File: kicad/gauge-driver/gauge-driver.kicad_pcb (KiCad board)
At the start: 2 copper layers, 18 parts, among them J1 Conn_01x02_Socket, U1 ESP32-WROOM-32E, U2 SN65HVD230, U3 LM2675M-3.3, Y1 Crystal

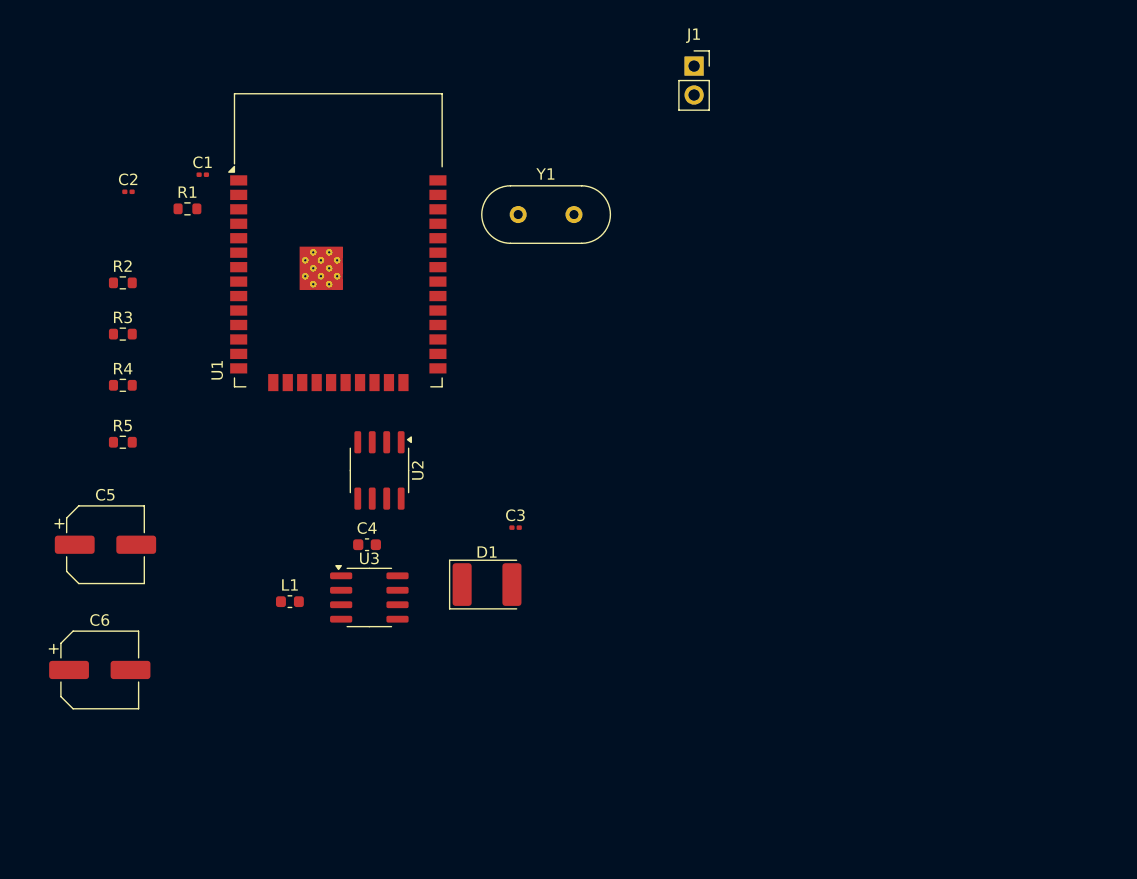
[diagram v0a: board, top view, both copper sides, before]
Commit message: kicad
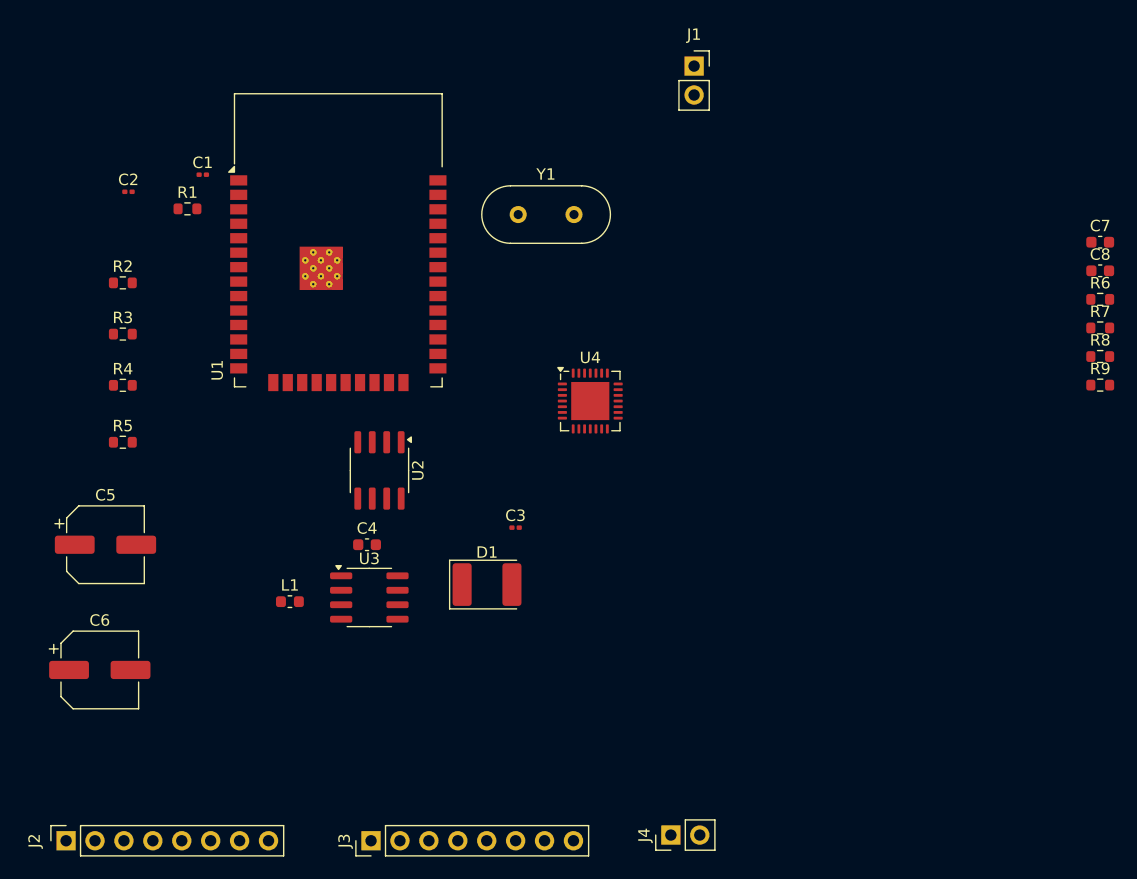
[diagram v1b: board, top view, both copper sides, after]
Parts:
- added C7: 4.7uF, Capacitor_SMD:C_0603_1608Metric, F.Cu at (106.2, 41.4)
- added C8: 4.7uF, Capacitor_SMD:C_0603_1608Metric, F.Cu at (106.2, 43.9)
- added J2: Conn_01x08, Connector_PinSocket_2.54mm:PinSocket_1x08_P2.54mm_Vertical, F.Cu at (15.3, 94.0)
- added J3: Conn_01x08, Connector_PinHeader_2.54mm:PinHeader_1x08_P2.54mm_Vertical, F.Cu at (42.1, 94.0)
- added J4: Conn_01x02_Socket, Connector_PinHeader_2.54mm:PinHeader_1x02_P2.54mm_Vertical, F.Cu at (68.5, 93.5)
- added R6: 10K, Resistor_SMD:R_0603_1608Metric, F.Cu at (106.2, 46.5)
- added R7: 2K, Resistor_SMD:R_0603_1608Metric, F.Cu at (106.2, 49.0)
- added R8: 22.1K, Resistor_SMD:R_0603_1608Metric, F.Cu at (106.2, 51.5)
- added R9: 47.5K, Resistor_SMD:R_0603_1608Metric, F.Cu at (106.2, 54.0)
- added U4: CP2102N-Axx-xQFN28, Package_DFN_QFN:QFN-28-1EP_5x5mm_P0.5mm_EP3.35x3.35mm, F.Cu at (61.4, 55.4)
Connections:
- C6 pad 1: /Vout_3v3 -> VDD33
- L1 pad 2: /Vout_3v3 -> VDD33
- U2 pad 3: VDD -> VDD33
- U3 pad 4: /Vout_3v3 -> VDD33

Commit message: Fixed re-ordering. Both screens now loading logo
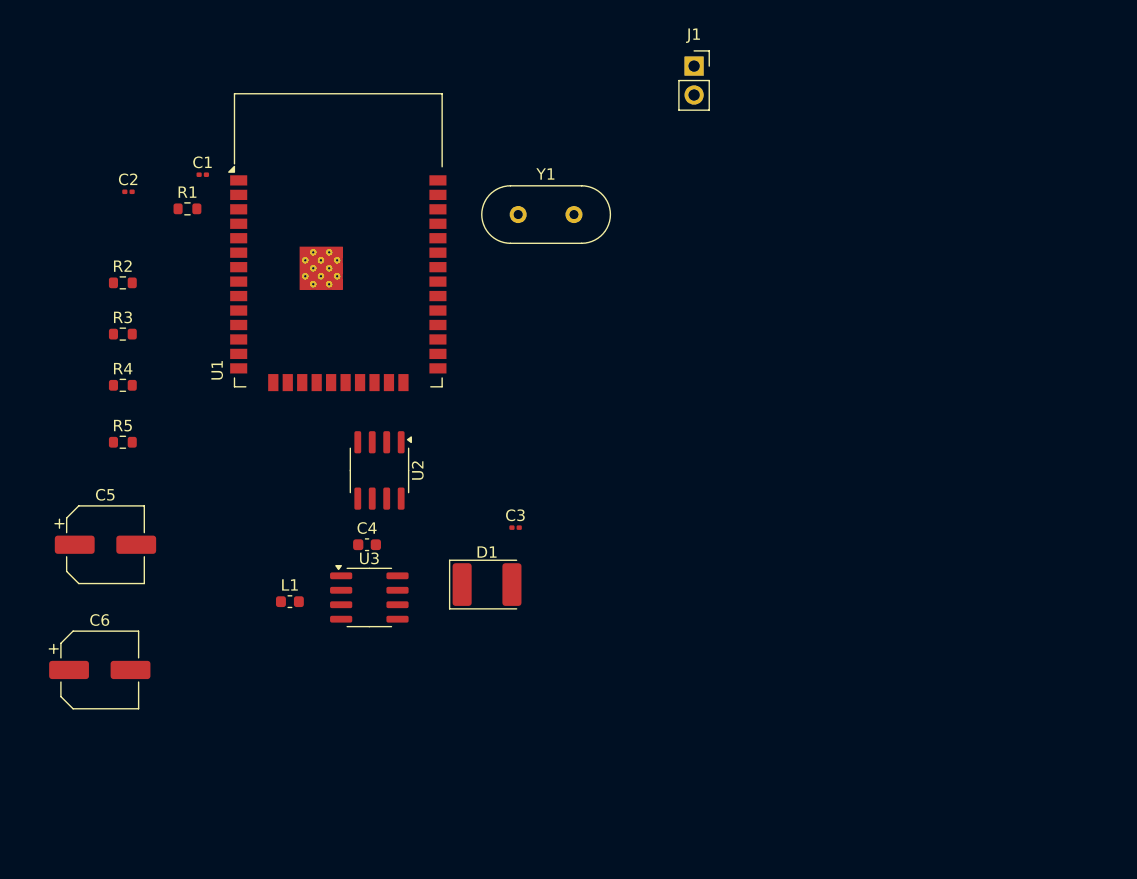
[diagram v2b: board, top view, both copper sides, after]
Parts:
- removed C7, C8: 4.7uF, Capacitor_SMD:C_0603_1608Metric
- removed J2: Conn_01x08, Connector_PinSocket_2.54mm:PinSocket_1x08_P2.54mm_Vertical
- removed J3: Conn_01x08, Connector_PinHeader_2.54mm:PinHeader_1x08_P2.54mm_Vertical
- removed J4: Conn_01x02_Socket, Connector_PinHeader_2.54mm:PinHeader_1x02_P2.54mm_Vertical
- removed R6: 10K, Resistor_SMD:R_0603_1608Metric
- removed R7: 2K, Resistor_SMD:R_0603_1608Metric
- removed R8: 22.1K, Resistor_SMD:R_0603_1608Metric
- removed R9: 47.5K, Resistor_SMD:R_0603_1608Metric
- removed U4: CP2102N-Axx-xQFN28, Package_DFN_QFN:QFN-28-1EP_5x5mm_P0.5mm_EP3.35x3.35mm
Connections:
- C6 pad 1: VDD33 -> /Vout_3v3
- L1 pad 2: VDD33 -> /Vout_3v3
- U2 pad 3: VDD33 -> VDD
- U3 pad 4: VDD33 -> /Vout_3v3
